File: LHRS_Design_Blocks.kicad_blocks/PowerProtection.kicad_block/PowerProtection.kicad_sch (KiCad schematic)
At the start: 17 parts, among them U7 LM76202QPWPRQ1

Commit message: UTSVT to LHRS
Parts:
- U7: footprint UTSVT_Power:LM76202QPWPRQ1 -> LHRS_Power:LM76202QPWPRQ1; symbol utsvt_power:LM76202QPWPRQ1 -> lhrs_power:LM76202QPWPRQ1
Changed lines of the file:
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@@
 	)
 	(symbol
-		(lib_id "utsvt_power:LM76202QPWPRQ1")
+		(lib_id "lhrs_power:LM76202QPWPRQ1")
 		(at 67.31 31.75 0)
 		(unit 1)
@@
 			)
 		)
-		(property "Footprint" "UTSVT_Power:LM76202QPWPRQ1"
+		(property "Footprint" "LHRS_Power:LM76202QPWPRQ1"
 			(at 93.98 126.67 0)
 			(effects

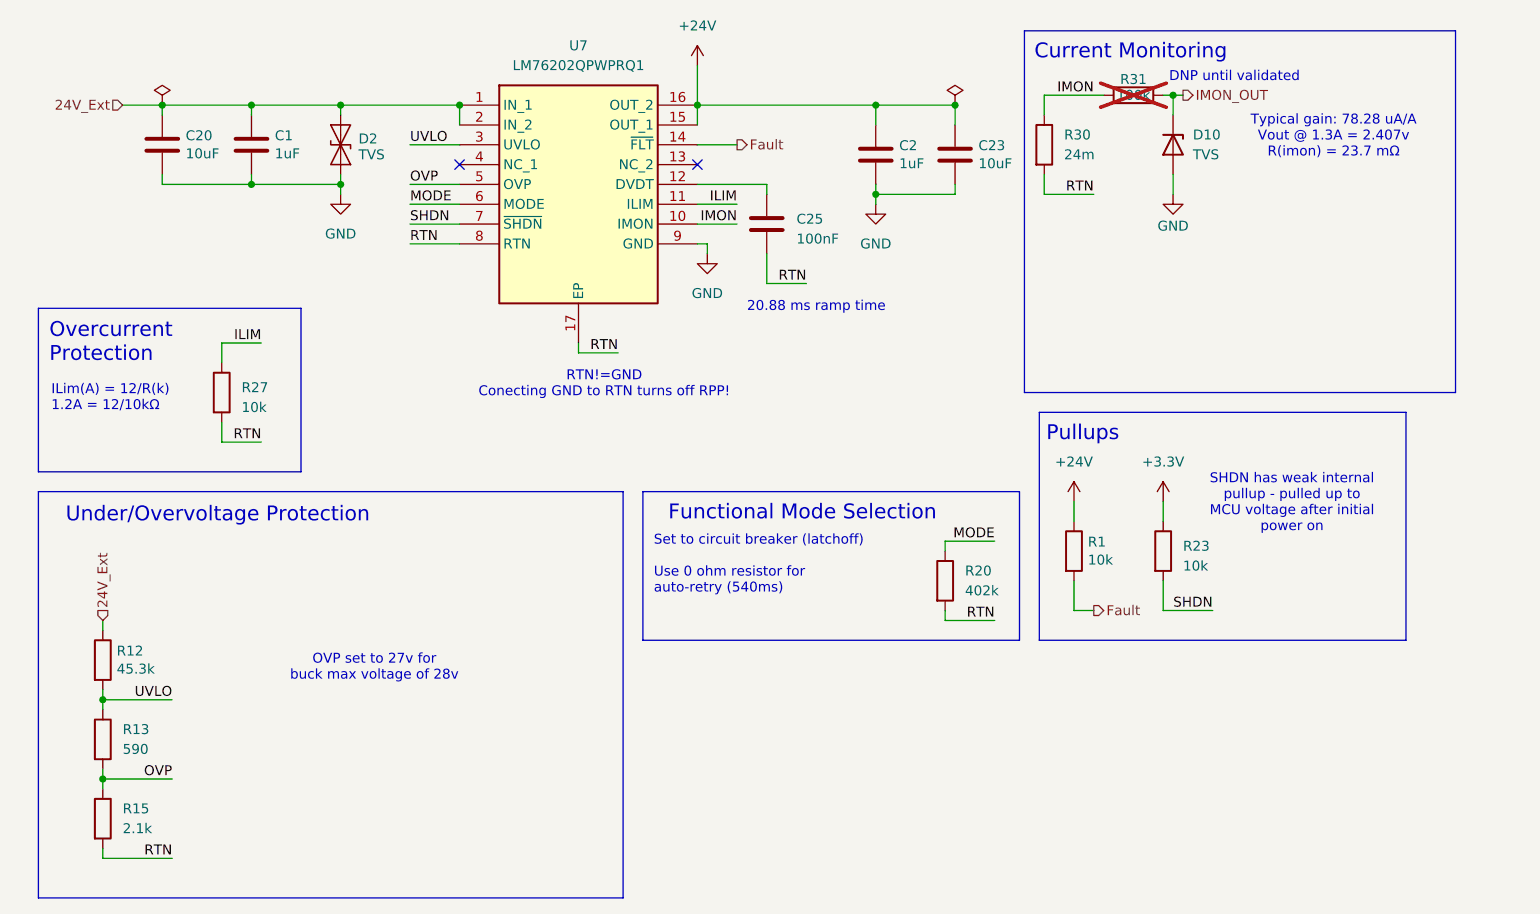
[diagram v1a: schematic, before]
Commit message: merged in pp and contactors
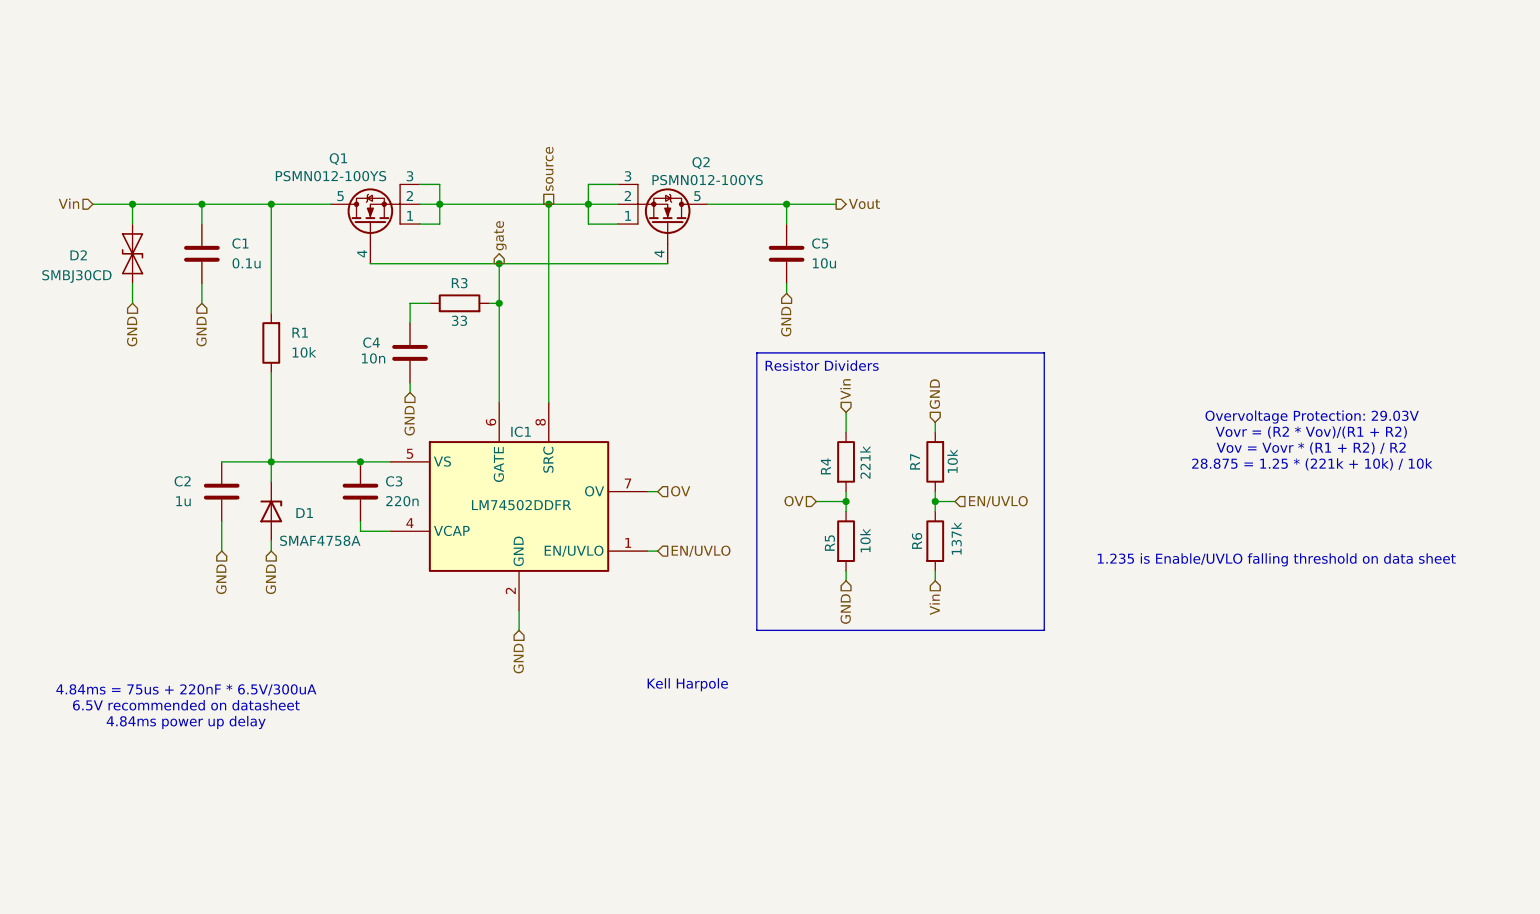
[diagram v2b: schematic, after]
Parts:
- removed C20, C23: 10uF, Capacitor_SMD:C_0805_2012Metric_Pad1.18x1.45mm_HandSolder, symbol Device:C
- removed C25: 100nF, Capacitor_SMD:C_0603_1608Metric_Pad1.08x0.95mm_HandSolder, symbol Device:C
- removed D10: TVS, Diode_SMD:D_SOD-123F, symbol Device:D_Zener
- removed D2: TVS, Diode_SMD:D_SOD-323_HandSoldering, symbol Diode:SD12_SOD323
- removed R12: 45.3k, Resistor_SMD:R_0603_1608Metric_Pad0.98x0.95mm_HandSolder, symbol Device:R
- removed R13: 590, Resistor_SMD:R_0603_1608Metric_Pad0.98x0.95mm_HandSolder, symbol Device:R
- removed R15: 2.1k, Resistor_SMD:R_0603_1608Metric_Pad0.98x0.95mm_HandSolder, symbol Device:R
- removed R20: 402k, Resistor_SMD:R_0603_1608Metric_Pad0.98x0.95mm_HandSolder, symbol Device:R
- removed R23, R27: 10k, Resistor_SMD:R_0603_1608Metric_Pad0.98x0.95mm_HandSolder, symbol Device:R
- removed R30: 24m, Resistor_SMD:R_0603_1608Metric_Pad0.98x0.95mm_HandSolder, symbol Device:R
- removed R31: 100k, Resistor_SMD:R_0603_1608Metric_Pad0.98x0.95mm_HandSolder, symbol Device:R
- removed U7: LM76202QPWPRQ1, LHRS_Power:LM76202QPWPRQ1, symbol lhrs_power:LM76202QPWPRQ1
- added C3: 220n, Capacitor_SMD:C_0603_1608Metric_Pad1.08x0.95mm_HandSolder, symbol Device:C
- added C4: 10n, Capacitor_SMD:C_0603_1608Metric_Pad1.08x0.95mm_HandSolder, symbol ECE319H:C
- added C5: 10u, Capacitor_SMD:C_0805_2012Metric_Pad1.18x1.45mm_HandSolder, symbol Device:C
- added D1: SMAF4758A, LHRS_Passives:SODFL5026X125N, symbol Device:D_Zener
- added D2: SMBJ30CD, Diode_SMD:D_SMB, symbol Device:D_Zener
- added IC1: LM74502DDFR, LHRS_Power:LM74502DDFR, symbol LHRS_ICs:LM74502HDDFR
- added Q1, Q2: PSMN012-100YS, Package_TO_SOT_SMD:LFPAK56, symbol lhrs_power:PSMN012-100YS
- added R3: 33, Resistor_SMD:R_0603_1608Metric_Pad0.98x0.95mm_HandSolder, symbol Device:R
- added R4: 221k, Resistor_SMD:R_0603_1608Metric_Pad0.98x0.95mm_HandSolder, symbol Device:R
- added R5, R7: 10k, Resistor_SMD:R_0603_1608Metric_Pad0.98x0.95mm_HandSolder, symbol Device:R
- added R6: 137k, Resistor_SMD:R_0603_1608Metric_Pad0.98x0.95mm_HandSolder, symbol Device:R
- C1: value 1uF -> 0.1u; LCSC P/N (none) -> C14663; P/N MLASU168SB5105KTNA01 -> MLASH168SB7104KTNA01
- C2: value 1uF -> 1u; LCSC P/N (none) -> C15849
- R1: LCSC P/N (none) -> C25804; Mouser Part Number (none) -> 71-CRCW060310K0FKEI; P/N CRCW060310K0FKEI -> CRCW060310K0FKEI
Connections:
- net Fault is gone; now on net Vin: R1.2
- net GND: now also C2.1, C4.2, C5.2, D1.2 (A), D2.2 (A2), IC1.2 (GND), R5.2, R7.2; no longer C2.2
- net +24V: no longer names the net of R1.1
- net +24V: now also C2.2, C3.1, D1.1 (K), IC1.5 (VS); no longer C2.1
- net 24V_Ext renamed Vin
- net Vin: now also D2.1 (A1), Q1.5, R4.1, R6.2
- new net: C3.2, IC1.4 (VCAP)
- new net: C4.1, R3.1
- new net EN/UVLO: IC1.1 (EN/UVLO), R6.1, R7.1
- new net OV: IC1.7 (OV), R4.2, R5.1
- new net Vout: C5.1, Q2.5
- new net gate: IC1.6 (GATE), Q1.4, Q2.4, R3.2
- new net source: IC1.8 (SRC), Q1.1, Q1.2, Q1.3, Q2.1, Q2.2, Q2.3
- no-connect marks 2 -> 0
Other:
- note added: "1.235 is Enable/UVLO falling threshold on data sheet"
- note added: "4.84ms = 75us + 220nF * 6.5V/300uA 6.5V recommended on datasheet 4.84ms power up delay"
- note added: "Kell Harpole"
- note added: "Overvoltage Protection: 29.03V Vovr = (R2 * Vov)/(R1 + R2) Vov = Vovr * (R1 + R2) / R2 28.875 = 1.25 * (221k + 10k) / 10k"
- note removed: "20.88 ms ramp time"
- note removed: "Current Monitoring"
- note removed: "DNP until validated"
- note removed: "Functional Mode Selection"
- note removed: "ILim(A) = 12/R(k) 1.2A = 12/10kΩ"
- note removed: "OVP set to 27v for buck max voltage of 28v"
- note removed: "Overcurrent Protection"
- note removed: "Pullups"
- note removed: "RTN!=GND Conecting GND to RTN turns off RPP!"
- note removed: "SHDN has weak internal pullup - pulled up to MCU voltage after initial power on"
- note removed: "Set to circuit breaker (latchoff) Use 0 ohm resistor for auto-retry (540ms)"
- note removed: "Typical gain: 78.28 uA/A Vout @ 1.3A = 2.407v R(imon) = 23.7 mΩ"
- note removed: "Under/Overvoltage Protection"
